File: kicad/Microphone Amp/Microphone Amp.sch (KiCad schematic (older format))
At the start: 24 parts, among them J1 Pad, J2 Pad, J4 Audio_Jack, M1 Electret, U3 LM358

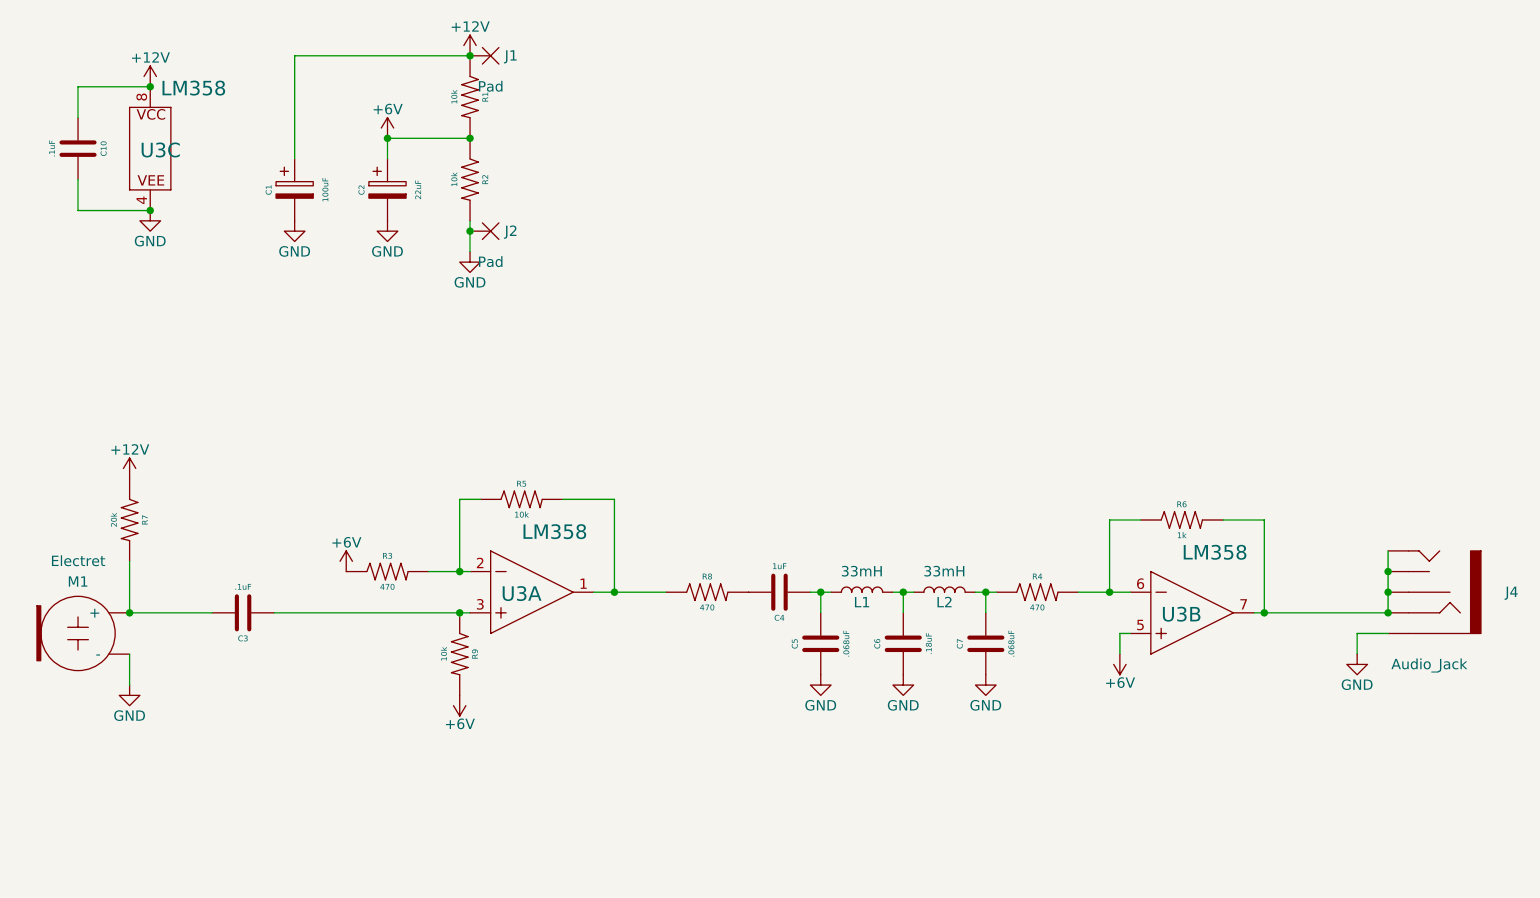
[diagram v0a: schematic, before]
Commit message: u
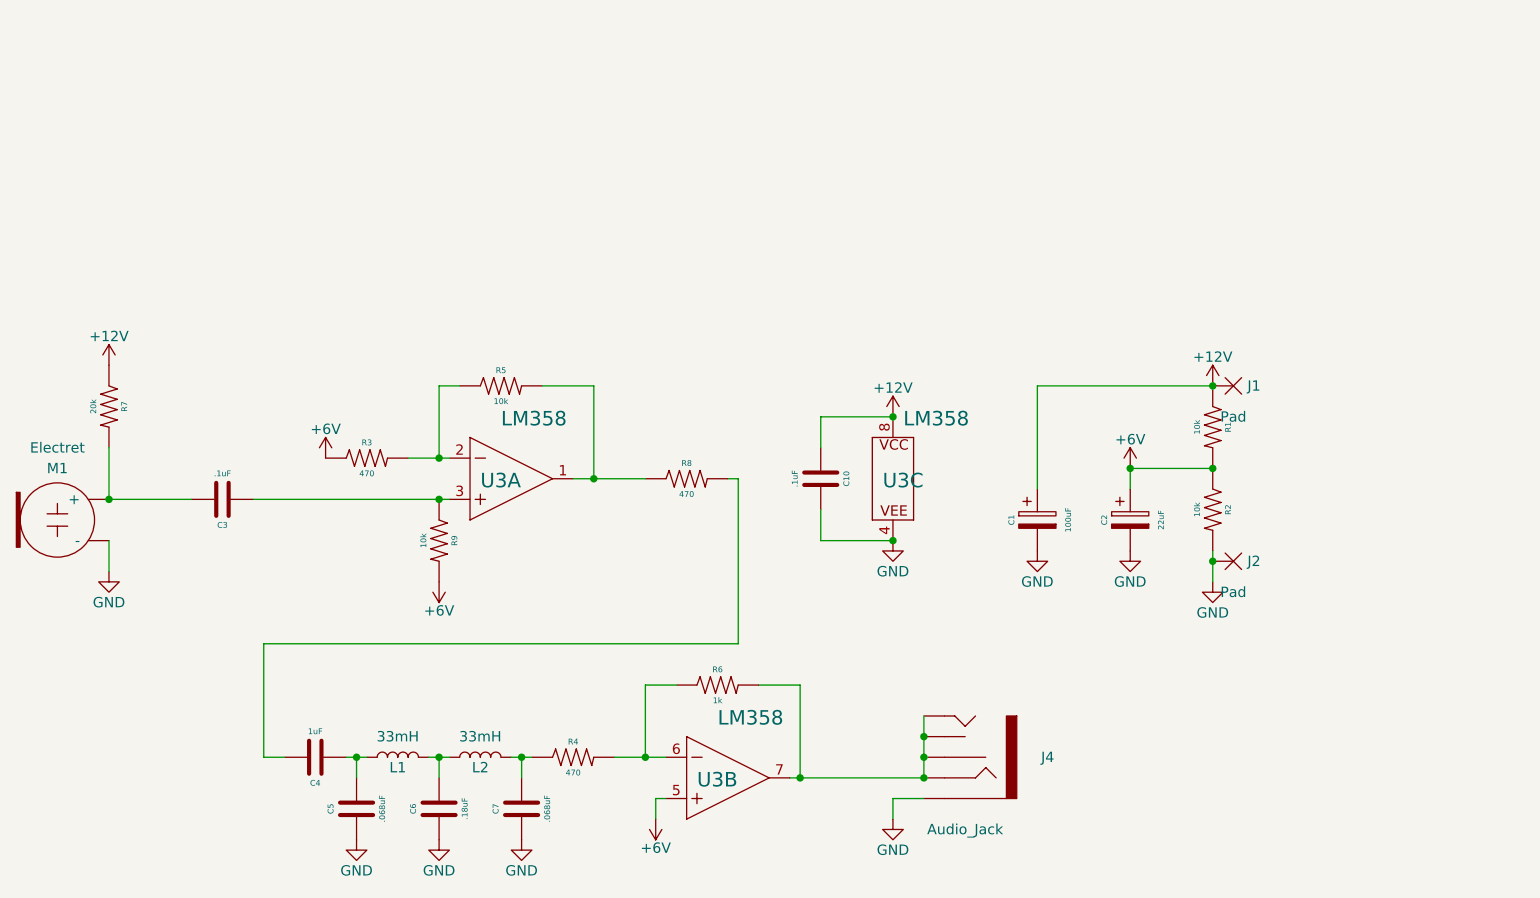
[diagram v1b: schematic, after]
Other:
- moved on the sheet: C1, C10, C2, C3, C4, C5, C6, C7, J1, J2, J4, L1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
